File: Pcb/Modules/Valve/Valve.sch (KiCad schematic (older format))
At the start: 19 parts, among them CON1 Valve1, CON2 Valve3, CON3 Power, CON4 Valve2, CON5 Valve4, J1 JACK_RJ45, P1 Servo1, P2 Servo2, Q1 Q_NMOS_GSD, Q2 Q_NMOS_GSD, Q3 Q_NMOS_GSD, Q4 Q_NMOS_GSD

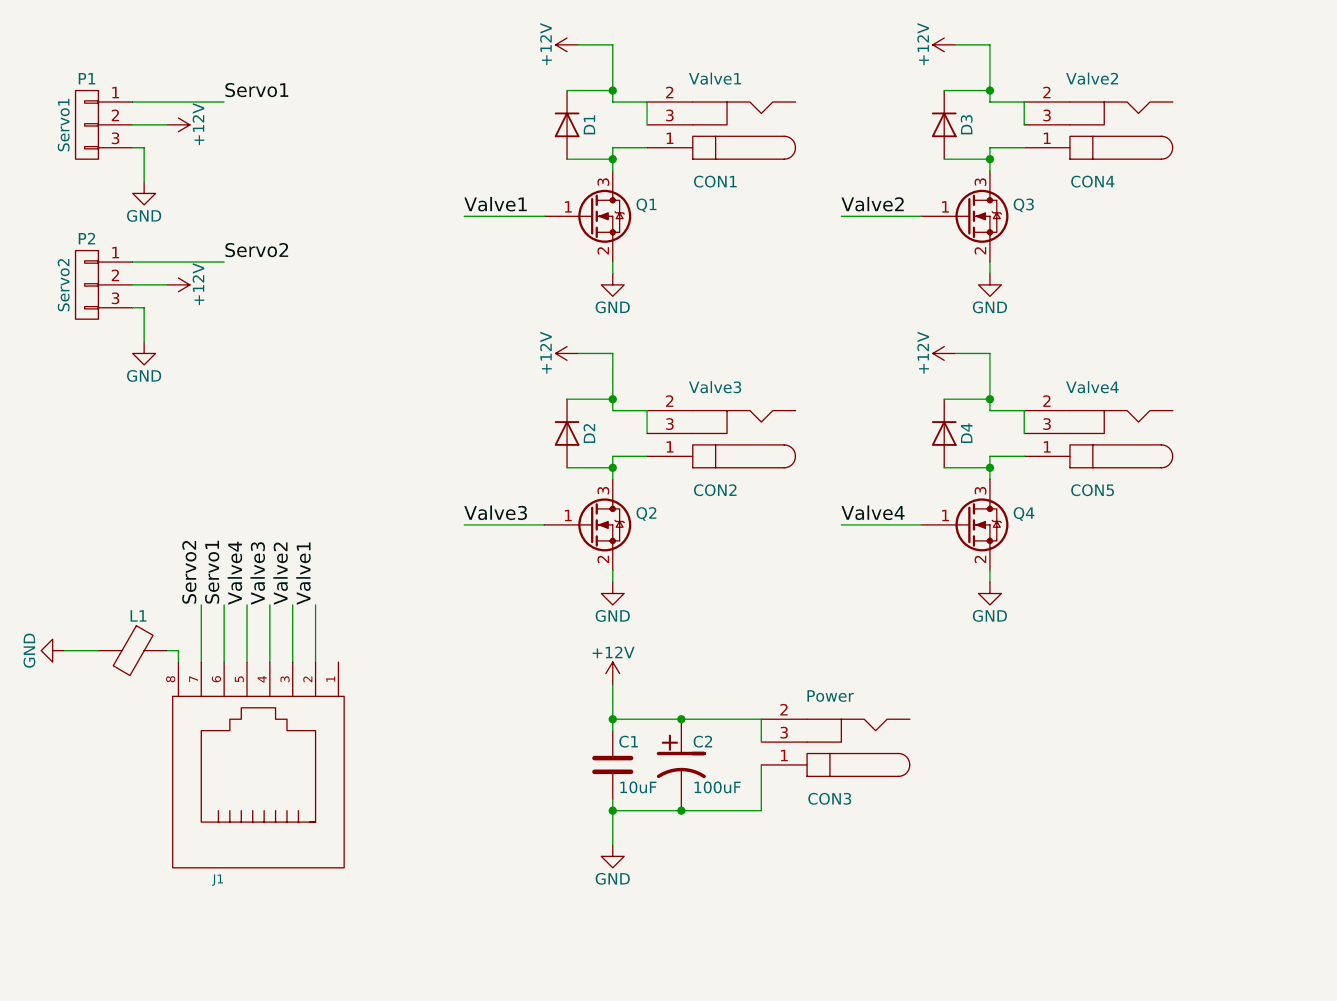
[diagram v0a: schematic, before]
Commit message: Update Valve module
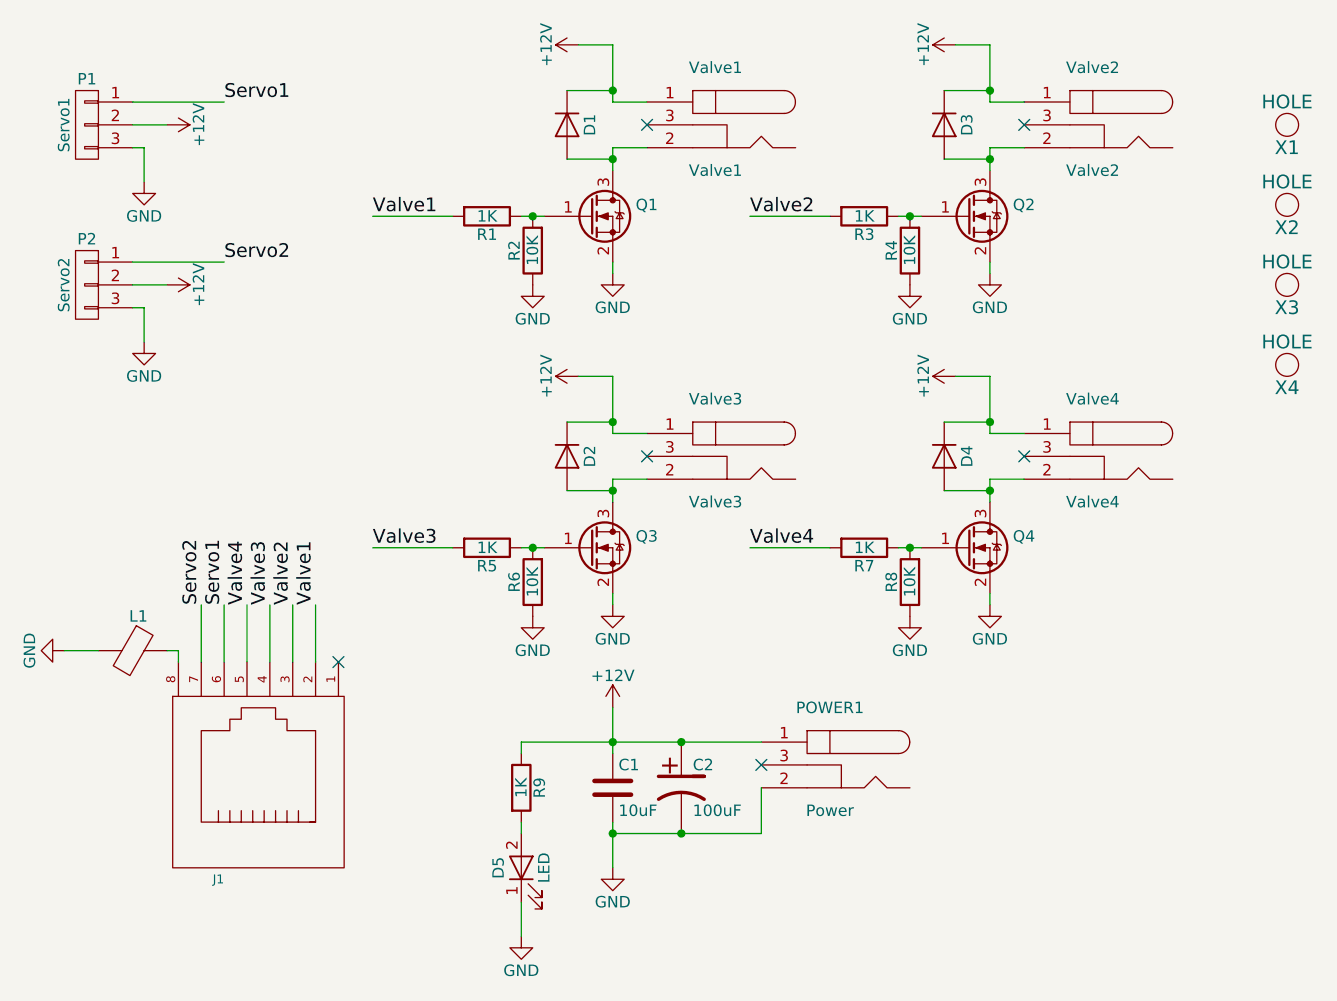
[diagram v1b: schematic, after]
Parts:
- added D5: LED, LEDs:LED_0805, symbol LED
- added R1, R3, R5, R7, R9: 1K, Resistors_SMD:R_0603, symbol R
- added R2, R4, R6, R8: 10K, Resistors_SMD:R_0603, symbol R
- added X1, X2, X3, X4: HOLE, Mounting_Holes:MountingHole_2.2mm_M2_ISO14580_Pad, symbol HOLE
- renumbered CON3 to POWER1, Q3 to Q2, Q2 to Q3, CON1 to Valve1, CON4 to Valve2, CON2 to Valve3, CON5 to Valve4
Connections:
- net +12V: now also POWER1.1, Valve1.1, Valve2.1, Valve3.1, Valve4.1, R9.1; no longer POWER1.2, POWER1.3, Valve1.2, Valve1.3, Valve2.2, Valve2.3, Valve3.2, Valve3.3, Valve4.2, Valve4.3
- net GND: now also POWER1.2, D5.1 (K), R2.1, R4.1, R6.1, R8.1; no longer POWER1.1
- net Valve1: now also R1.2; no longer Q1.1 (G)
- net Valve2: now also R3.2; no longer Q2.1 (G)
- net Valve3: now also R5.2; no longer Q3.1 (G)
- net Valve4: now also R7.2; no longer Q4.1 (G)
- net at D1.2 (A), Q1.3 (D): now also Valve1.2; no longer Valve1.1
- net at D3.2 (A), Q2.3 (D): now also Valve2.2; no longer Valve2.1
- net at D2.2 (A), Q3.3 (D): now also Valve3.2; no longer Valve3.1
- net at D4.2 (A), Q4.3 (D): now also Valve4.2; no longer Valve4.1
- new net: Q1.1 (G), R1.1, R2.2
- new net: Q2.1 (G), R3.1, R4.2
- new net: Q3.1 (G), R5.1, R6.2
- new net: Q4.1 (G), R7.1, R8.2
- new net: D5.2 (A), R9.2
- no-connect marks 0 -> 6
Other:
- moved on the sheet: C1, C2, D2, D4, POWER1, Q3, Q4, Valve3, Valve4
